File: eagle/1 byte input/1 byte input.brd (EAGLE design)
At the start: 82.5 x 50.5 mm, 13 parts, among them IC1 74LS595N, IC2 74LS595N, X1 MKDSN1,5/8-5,08, X2 MKDSN1,5/8-5,08, X3 MKDSN1,5/5-5,08, X4 MKDSN1,5/5-5,08, X5 MKDSN1,5/2-5,08

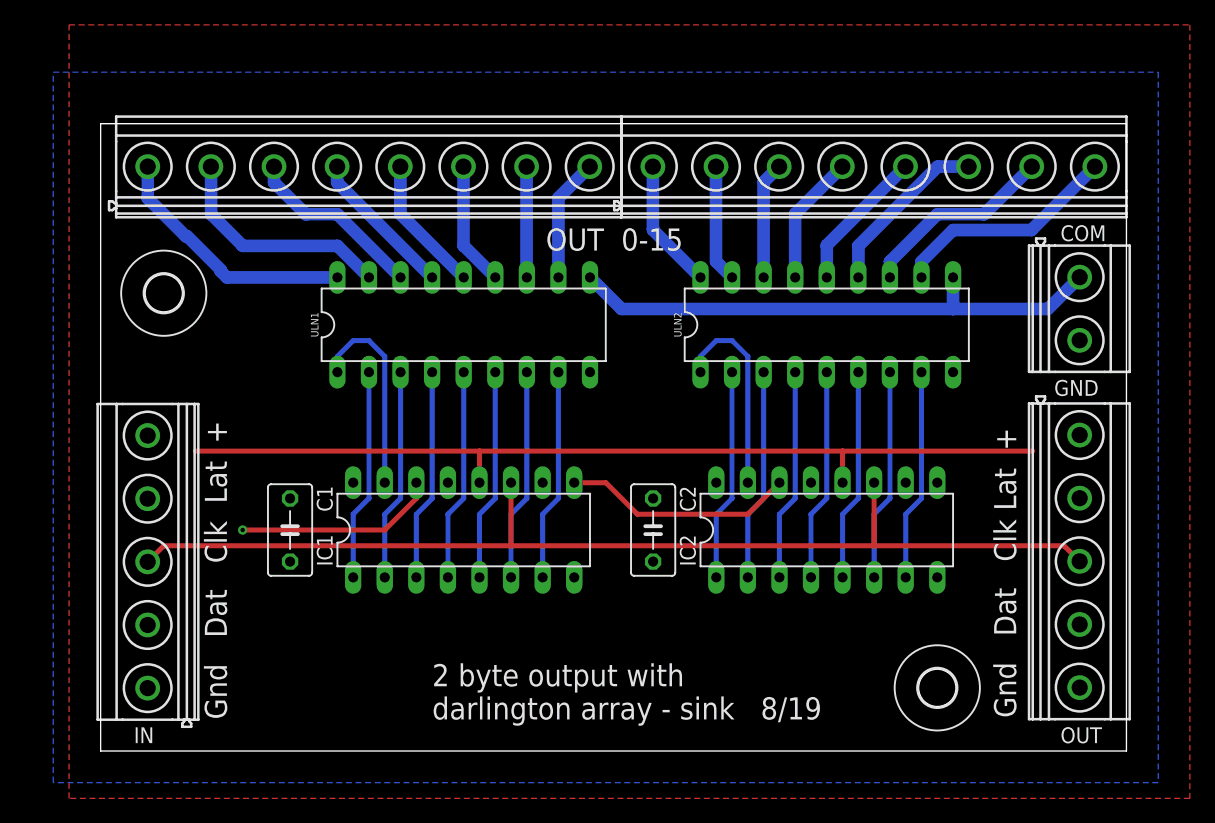
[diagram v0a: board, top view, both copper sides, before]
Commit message: periodic check in - everything working so far with breadboards.
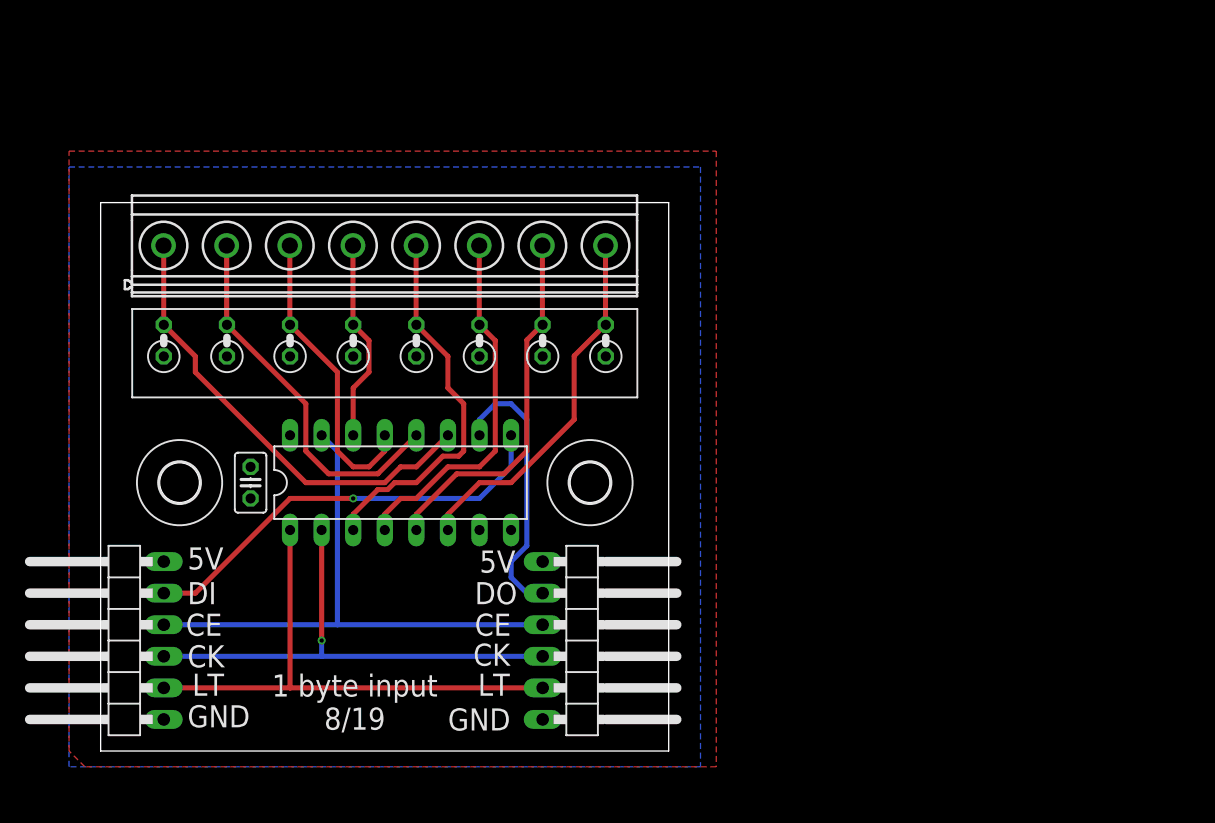
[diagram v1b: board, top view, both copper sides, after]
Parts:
- removed C2: (no value), resistor:C050-035X075
- removed IC2: 74LS595N, 74xx-us:DIL16
- removed ULN1, ULN2: (no value), SparkFun-IC-Special-Function:DIL18
- removed X1, X2: MKDSN1,5/8-5,08, con-phoenix-508:MKDSN1,5/8-5,08
- removed X4: MKDSN1,5/5-5,08, con-phoenix-508:MKDSN1,5/5-5,08
- removed X5: MKDSN1,5/2-5,08, con-phoenix-508:MKDSN1,5/2-5,08
- added JP1, JP2: (no value), pinhead:1X06/90
- added R1, R2, R3, R4, R5, R6, R7, R8: (no value), resistor:0207/2V
- C1: value (none) -> 0.1uf; device resistor:C050-035X075 -> resistor:C025-025X050
- H1, H2: value MOUNT-HOLE3.0 -> MOUNT-HOLE3.2; device holes:3,0 -> holes:3,2
- IC1: value 74LS595N -> 74LS165N
- X3: value MKDSN1,5/5-5,08 -> MKDSN1,5/8-5,08; device con-phoenix-508:MKDSN1,5/5-5,08 -> con-phoenix-508:MKDSN1,5/8-5,08
- moved H2 32.5 mm to (39.4, 21.6)
- moved X3 31.8 mm to (22.9, 40.6), turned to 0 degrees
- moved H1 15.3 mm to (6.35, 21.6)
- moved IC1 6.35 mm to (24.1, 21.6)
- moved C1 4.96 mm to (12.1, 21.6)
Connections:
- removed net COM: ULN1.10, ULN2.10, X5.1
- removed net DI: IC1.14, X3.4
- removed net DO: IC2.9, X4.2
- removed net DP: IC1.9, IC2.14
- removed net N$1: ULN1.18, X1.1
- removed net N$10: ULN2.17, X2.2
- removed net N$11: ULN2.16, X2.3
- removed net N$12: ULN2.15, X2.4
- removed net N$13: ULN2.14, X2.5
- removed net N$14: ULN2.13, X2.6
- removed net N$15: ULN2.12, X2.7
- removed net N$16: ULN2.11, X2.8
- removed net N$2: ULN1.17, X1.2
- removed net N$3: ULN1.16, X1.3
- removed net N$4: ULN1.15, X1.4
- removed net N$5: ULN1.14, X1.5
- removed net N$6: ULN1.13, X1.6
- removed net N$7: ULN1.12, X1.7
- removed net N$8: ULN1.11, X1.8
- removed net N$9: ULN2.18, X2.1
- removed net OUT0: IC1.15, ULN1.1
- removed net OUT1: IC1.1, ULN1.2
- removed net OUT10: IC2.2, ULN2.3
- removed net OUT11: IC2.3, ULN2.4
- removed net OUT12: IC2.4, ULN2.5
- removed net OUT13: IC2.5, ULN2.6
- removed net OUT14: IC2.6, ULN2.7
- removed net OUT15: IC2.7, ULN2.8
- removed net OUT2: IC1.2, ULN1.3
- removed net OUT3: IC1.3, ULN1.4
- removed net OUT4: IC1.4, ULN1.5
- removed net OUT5: IC1.5, ULN1.6
- removed net OUT6: IC1.6, ULN1.7
- removed net OUT7: IC1.7, ULN1.8
- removed net OUT8: IC2.15, ULN2.1
- removed net OUT9: IC2.1, ULN2.2
- removed net VCC: C1.1, C2.1, IC1.10, IC1.16, IC2.10, IC2.16, X3.5, X4.1
- new net +5V: C1.1, IC1.16, JP1.6, JP2.1, R1.1, R2.1, R3.1, R4.1, R5.1, R6.1, R7.1, R8.1
- new net CE: IC1.15, JP1.4, JP2.3
- new net INA0: IC1.11, R1.2, X3.1
- new net INA1: IC1.12, R2.2, X3.2
- new net INA2: IC1.13, R3.2, X3.3
- new net INA3: IC1.14, R4.2, X3.4
- new net INA4: IC1.3, R5.2, X3.5
- new net INA5: IC1.4, R6.2, X3.6
- new net INA6: IC1.5, R7.2, X3.7
- new net INA7: IC1.6, R8.2, X3.8
- new net S0: IC1.9, JP1.5
- new net S1: IC1.10, JP2.2
- net CLK: now also IC1.2, JP1.3, JP2.4; no longer IC1.11, IC2.11, X3.3, X4.3
- net GND: now also JP1.1, JP2.6; no longer C2.2, IC1.13, IC2.13, IC2.8, ULN1.9, ULN2.9, X3.1, X4.5, X5.2
- net LATCH: now also IC1.1, JP1.2, JP2.5; no longer IC1.12, IC2.12, X3.2, X4.4
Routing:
- net CE: track 0.00 -> 46.2 mm
- net CLK: track 86.2 -> 40.6 mm, vias 0 -> 1
- net COM: track 44.0 -> 0.00 mm
- net INA0: track 0.00 -> 36.8 mm
- net S0: track 0.00 -> 34.7 mm, vias 0 -> 1
- net INA4: track 0.00 -> 30.4 mm
- net INA1: track 0.00 -> 30.1 mm
- net INA7: track 0.00 -> 29.7 mm
- net INA6: track 0.00 -> 29.3 mm
- net INA5: track 0.00 -> 29.3 mm
- net LATCH: track 72.4 -> 43.2 mm
- net INA2: track 0.00 -> 24.3 mm
- net S1: track 0.00 -> 22.4 mm
- net N$1: track 20.5 -> 0.00 mm
- net N$2: track 18.6 -> 0.00 mm
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- added copper zone on layer 1, net +5V
- removed copper zone on layer 1, net VCC
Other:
- board size 82.5 x 50.5 mm -> 45.7 x 44.1 mm
- board text added: "1 byte input 8/19"
- board text added: "5V"
- board text added: "CE"
- board text added: "CK"
- board text added: "DI"
- board text added: "DO"
- board text added: "LT"
- board text removed: "2 byte output with darlington array - sink 8/19"
- board text removed: "COM"
- board text removed: "Gnd Dat Clk Lat +"
- board text removed: "IN"
- board text removed: "OUT"
- board text removed: "OUT 0-15"
